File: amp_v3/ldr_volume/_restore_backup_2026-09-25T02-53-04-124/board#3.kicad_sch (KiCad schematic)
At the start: 56 parts, among them J12 EXT, J16 CTRL, J17 CTRL, J19 PWR_IN, J20 I2C_L, J21 I2C_R, J23 MUTE, J37 MUTE, J39 UART, J45 MUTE_OUT, Q1 BC547, Q11 2N7000, Q12 2N7000, Q14 BC547, Q2 BC557, Q3 BC547, Q4 BC557, Q5 BC547, Q6 BC557, Q7 BC547, Q8 BC557, U4 4N25

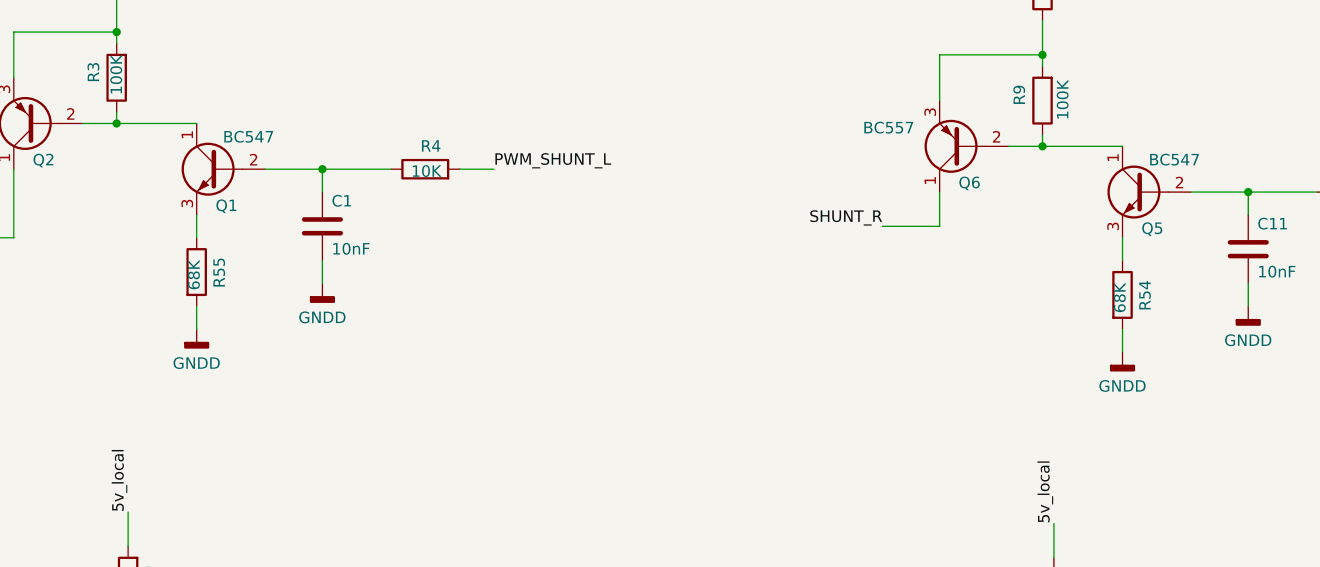
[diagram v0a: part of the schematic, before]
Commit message: updates
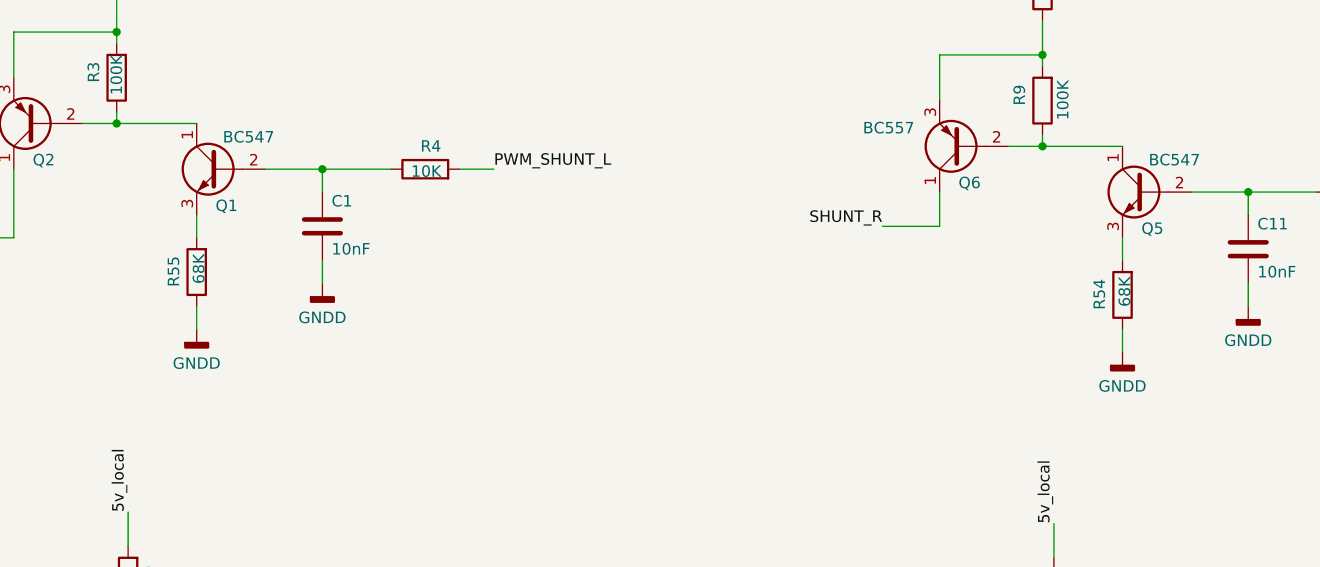
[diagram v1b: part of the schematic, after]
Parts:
- R54, R55: footprint Resistor_THT:R_Axial_DIN0309_L9.0mm_D3.2mm_P2.54mm_Vertical -> Resistor_THT:R_Axial_DIN0207_L6.3mm_D2.5mm_P7.62mm_Horizontal
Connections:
- net GNDD: now also R54.1, R55.1; no longer R54.2, R55.2
- net at Q1.3 (E): now also R55.2; no longer R55.1
- net at Q5.3 (E): now also R54.2; no longer R54.1
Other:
- moved on the sheet: R54, R55
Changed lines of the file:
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@@
 	(symbol
 		(lib_id "Device:R")
-		(at 132.08 -226.06 0)
+		(at 132.08 -226.06 180)
 		(unit 1)
 		(body_style 1)
@@
 		(dnp no)
 		(property "Reference" "R54"
-			(at 134.62 -224.282 90)
+			(at 129.54 -227.838 90)
 			(show_name no)
 			(do_not_autoplace no)
@@
 		)
 		(property "Value" "68K"
-			(at 131.826 -224.028 90)
-			(show_name no)
-			(do_not_autoplace no)
-			(effects
-				(font
-					(size 1.27 1.27)
-				)
-				(justify left)
-			)
-		)
-		(property "Footprint" "Resistor_THT:R_Axial_DIN0309_L9.0mm_D3.2mm_P2.54mm_Vertical"
-			(at 130.302 -226.06 90)
+			(at 132.334 -228.092 90)
+			(show_name no)
+			(do_not_autoplace no)
+			(effects
+				(font
+					(size 1.27 1.27)
+				)
+				(justify left)
+			)
+		)
+		(property "Footprint" "Resistor_THT:R_Axial_DIN0207_L6.3mm_D2.5mm_P7.62mm_Horizontal"
+			(at 133.858 -226.06 90)
 			(hide yes)
 			(show_name no)
@@
 	(symbol
 		(lib_id "Device:R")
-		(at 29.21 -228.6 0)
+		(at 29.21 -228.6 180)
 		(unit 1)
 		(body_style 1)
@@
 		(dnp no)
 		(property "Reference" "R55"
-			(at 31.75 -226.822 90)
+			(at 26.67 -230.378 90)
 			(show_name no)
 			(do_not_autoplace no)
@@
 		)
 		(property "Value" "68K"
-			(at 28.956 -226.568 90)
-			(show_name no)
-			(do_not_autoplace no)
-			(effects
-				(font
-					(size 1.27 1.27)
-				)
-				(justify left)
-			)
-		)
-		(property "Footprint" "Resistor_THT:R_Axial_DIN0309_L9.0mm_D3.2mm_P2.54mm_Vertical"
-			(at 27.432 -228.6 90)
-			(hide yes)
-			(show_name no)
+			(at 29.464 -230.632 90)
+			(show_name no)
+			(do_not_autoplace no)
+			(effects
+				(font
+					(size 1.27 1.27)
+				)
+				(justify left)
+			)
+		)
+		(property "Footprint" "Resistor_THT:R_Axial_DIN0207_L6.3mm_D2.5mm_P7.62mm_Horizontal"
+			(at 30.988 -228.6 90)
+			(hide yes)
+			(show_name no)
